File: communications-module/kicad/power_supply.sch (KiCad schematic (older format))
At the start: 25 parts, among them J1 IDC12, P2 USB_A, P3 USB_A, P4 USB_A, P5 BACKUP, U3 TPS2064, U4 PWR_CONN, U5 TPS2064

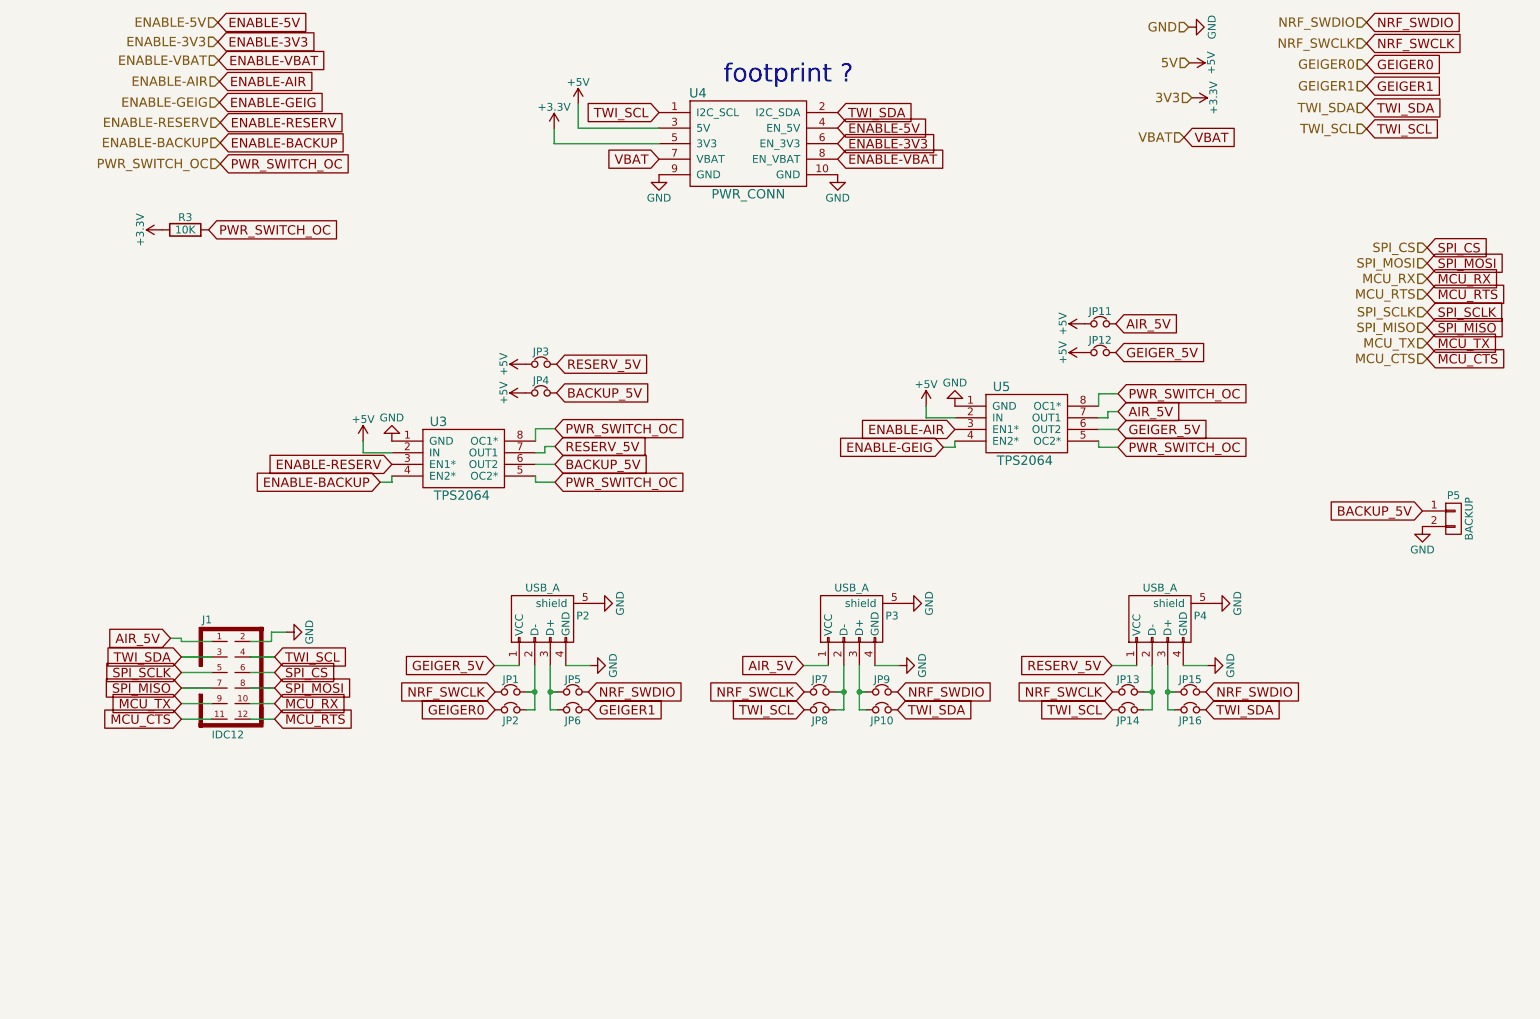
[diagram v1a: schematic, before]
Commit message: Communications Module schematic update
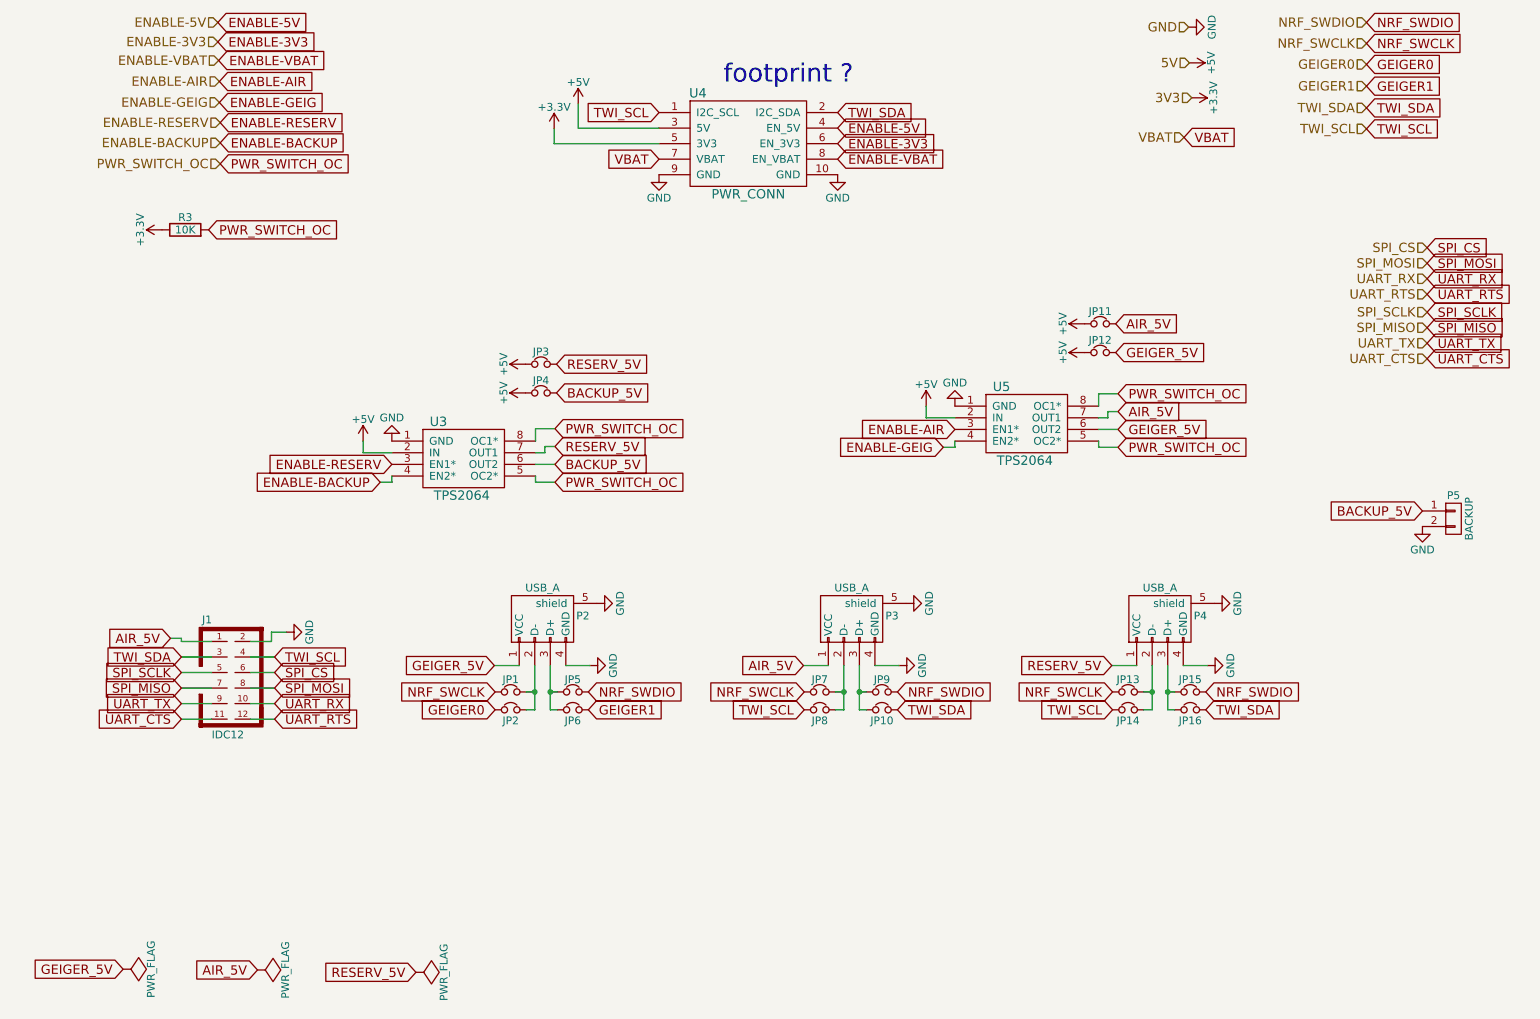
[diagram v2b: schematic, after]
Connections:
- net MCU_CTS renamed UART_CTS
- net MCU_RTS renamed UART_RTS
- net MCU_RX renamed UART_RX
- net MCU_TX renamed UART_TX
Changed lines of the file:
@@
 TWI_SDA
 $Comp
-L GND #PWR019
+L GND #PWR041
 U 1 1 589845A1
 P 4785 2270
-F 0 "#PWR019" H 4785 2020 50  0001 C CNN
+F 0 "#PWR041" H 4785 2020 50  0001 C CNN
 F 1 "GND" H 4785 2120 50  0000 C CNN
 F 2 "" H 4785 2270 60  0000 C CNN
@@
 $EndComp
 $Comp
-L GND #PWR020
+L GND #PWR042
 U 1 1 589845A7
 P 5935 2270
-F 0 "#PWR020" H 5935 2020 50  0001 C CNN
+F 0 "#PWR042" H 5935 2020 50  0001 C CNN
 F 1 "GND" H 5935 2120 50  0000 C CNN
 F 2 "" H 5935 2270 60  0000 C CNN
@@
 $EndComp
 $Comp
-L GND #PWR021
+L GND #PWR043
 U 1 1 589859EA
 P 6375 5030
-F 0 "#PWR021" H 6375 4780 50  0001 C CNN
+F 0 "#PWR043" H 6375 4780 50  0001 C CNN
 F 1 "GND" H 6375 4880 50  0000 C CNN
 F 2 "" H 6375 5030 60  0000 C CNN
@@
 $EndComp
 $Comp
-L GND #PWR022
+L GND #PWR044
 U 1 1 589859F7
 P 8315 5430
-F 0 "#PWR022" H 8315 5180 50  0001 C CNN
+F 0 "#PWR044" H 8315 5180 50  0001 C CNN
 F 1 "GND" H 8315 5280 50  0000 C CNN
 F 2 "" H 8315 5430 60  0000 C CNN
@@
 $EndComp
 $Comp
-L GND #PWR023
+L GND #PWR045
 U 1 1 58985A1D
 P 8360 5030
-F 0 "#PWR023" H 8360 4780 50  0001 C CNN
+F 0 "#PWR045" H 8360 4780 50  0001 C CNN
 F 1 "GND" H 8360 4880 50  0000 C CNN
 F 2 "" H 8360 5030 60  0000 C CNN
@@
 $EndComp
 $Comp
-L GND #PWR024
+L GND #PWR046
 U 1 1 58985A2A
 P 4340 5430
-F 0 "#PWR024" H 4340 5180 50  0001 C CNN
+F 0 "#PWR046" H 4340 5180 50  0001 C CNN
 F 1 "GND" H 4340 5280 50  0000 C CNN
 F 2 "" H 4340 5430 60  0000 C CNN
@@
 $EndComp
 $Comp
-L GND #PWR025
+L GND #PWR047
 U 1 1 58985A50
 P 4385 5030
-F 0 "#PWR025" H 4385 4780 50  0001 C CNN
+F 0 "#PWR047" H 4385 4780 50  0001 C CNN
 F 1 "GND" H 4385 4880 50  0000 C CNN
 F 2 "" H 4385 5030 60  0000 C CNN
@@
 $EndComp
 $Comp
-L GND #PWR026
+L GND #PWR048
 U 1 1 58985A5D
 P 6690 3760
-F 0 "#PWR026" H 6690 3510 50  0001 C CNN
+F 0 "#PWR048" H 6690 3510 50  0001 C CNN
 F 1 "GND" H 6690 3610 50  0000 C CNN
 F 2 "" H 6690 3760 60  0000 C CNN
@@
 	7615 4025 7740 4025
 $Comp
-L GND #PWR027
+L GND #PWR049
 U 1 1 58985A8F
 P 3065 3985
-F 0 "#PWR027" H 3065 3735 50  0001 C CNN
+F 0 "#PWR049" H 3065 3735 50  0001 C CNN
 F 1 "GND" H 3065 3835 50  0000 C CNN
 F 2 "" H 3065 3985 60  0000 C CNN
@@
 RESERV_5V
 $Comp
-L GND #PWR028
+L GND #PWR050
 U 1 1 58985AAE
 P 6330 5430
-F 0 "#PWR028" H 6330 5180 50  0001 C CNN
+F 0 "#PWR050" H 6330 5180 50  0001 C CNN
 F 1 "GND" H 6330 5280 50  0000 C CNN
 F 2 "" H 6330 5430 60  0000 C CNN
@@
 $EndComp
 $Comp
-L +5V #PWR029
+L +5V #PWR051
 U 1 1 58985ABE
 P 3925 3490
-F 0 "#PWR029" H 3925 3340 50  0001 C CNN
+F 0 "#PWR051" H 3925 3340 50  0001 C CNN
 F 1 "+5V" H 3925 3630 50  0000 C CNN
 F 2 "" H 3925 3490 60  0000 C CNN
@@
 $EndComp
 $Comp
-L +5V #PWR030
+L +5V #PWR052
 U 1 1 58985AD9
 P 7525 3230
-F 0 "#PWR030" H 7525 3080 50  0001 C CNN
+F 0 "#PWR052" H 7525 3080 50  0001 C CNN
 F 1 "+5V" H 7525 3370 50  0000 C CNN
 F 2 "" H 7525 3230 60  0000 C CNN
@@
 $EndComp
 $Comp
-L +5V #PWR031
+L +5V #PWR053
 U 1 1 58985AE6
 P 7525 3415
-F 0 "#PWR031" H 7525 3265 50  0001 C CNN
+F 0 "#PWR053" H 7525 3265 50  0001 C CNN
 F 1 "+5V" H 7525 3555 50  0000 C CNN
 F 2 "" H 7525 3415 60  0000 C CNN
@@
 5V
 $Comp
-L +5V #PWR032
+L +5V #PWR054
 U 1 1 58988CC2
 P 8200 1550
-F 0 "#PWR032" H 8200 1400 50  0001 C CNN
+F 0 "#PWR054" H 8200 1400 50  0001 C CNN
 F 1 "+5V" H 8200 1690 50  0000 C CNN
 F 2 "" H 8200 1550 60  0000 C CNN
@@
 $EndComp
 $Comp
-L +3.3V #PWR033
+L +3.3V #PWR055
 U 1 1 58989B65
 P 8215 1775
-F 0 "#PWR033" H 8215 1625 50  0001 C CNN
+F 0 "#PWR055" H 8215 1625 50  0001 C CNN
 F 1 "+3.3V" H 8215 1915 50  0000 C CNN
 F 2 "" H 8215 1775 60  0000 C CNN
@@
 TWI_SCL
 $Comp
-L +5V #PWR034
+L +5V #PWR056
 U 1 1 589845B4
 P 4265 1815
-F 0 "#PWR034" H 4265 1665 50  0001 C CNN
+F 0 "#PWR056" H 4265 1665 50  0001 C CNN
 F 1 "+5V" H 4265 1955 50  0000 C CNN
 F 2 "" H 4265 1815 60  0000 C CNN
@@
 $EndComp
 $Comp
-L +3.3V #PWR035
+L +3.3V #PWR057
 U 1 1 589845AE
 P 4110 1975
-F 0 "#PWR035" H 4110 1825 50  0001 C CNN
+F 0 "#PWR057" H 4110 1825 50  0001 C CNN
 F 1 "+3.3V" H 4110 2115 50  0000 C CNN
 F 2 "" H 4110 1975 60  0000 C CNN
@@
 BACKUP_5V
 $Comp
-L GND #PWR036
+L GND #PWR058
 U 1 1 589977EF
 P 9700 4535
-F 0 "#PWR036" H 9700 4285 50  0001 C CNN
+F 0 "#PWR058" H 9700 4285 50  0001 C CNN
 F 1 "GND" H 9700 4385 50  0000 C CNN
 F 2 "" H 9700 4535 60  0000 C CNN
@@
 AIR_5V
 $Comp
-L GND #PWR037
+L GND #PWR059
 U 1 1 58A00F9B
 P 8195 1320
-F 0 "#PWR037" H 8195 1070 50  0001 C CNN
+F 0 "#PWR059" H 8195 1070 50  0001 C CNN
 F 1 "GND" H 8195 1170 50  0000 C CNN
 F 2 "" H 8195 1320 60  0000 C CNN
@@
 $EndComp
 $Comp
-L +3.3V #PWR038
+L +3.3V #PWR060
 U 1 1 58999FE9
 P 1585 2625
-F 0 "#PWR038" H 1585 2475 50  0001 C CNN
+F 0 "#PWR060" H 1585 2475 50  0001 C CNN
 F 1 "+3.3V" H 1585 2765 50  0000 C CNN
 F 2 "" H 1585 2625 60  0000 C CNN
@@
 SPI_SCLK
 $Comp
-L GND #PWR039
+L GND #PWR061
 U 1 1 58A15D45
 P 2385 5215
-F 0 "#PWR039" H 2385 4965 50  0001 C CNN
+F 0 "#PWR061" H 2385 4965 50  0001 C CNN
 F 1 "GND" H 2385 5065 50  0000 C CNN
 F 2 "" H 2385 5215 60  0000 C CNN
@@
 	1905 5775 1710 5775
 Text GLabel 1710 5675 0    60   Input ~ 0
-MCU_TX
+UART_TX
 Text GLabel 2310 5675 2    60   Input ~ 0
-MCU_RX
+UART_RX
 Text GLabel 1710 5775 0    60   Input ~ 0
-MCU_CTS
+UART_CTS
 Text GLabel 2310 5775 2    60   Input ~ 0
-MCU_RTS
+UART_RTS
 Wire Wire Line
 	2155 5375 2310 5375
@@
 SPI_SCLK
 Text GLabel 9730 3355 2    60   Input ~ 0
-MCU_TX
+UART_TX
 Text GLabel 9730 3455 2    60   Input ~ 0
-MCU_CTS
+UART_CTS
 Text GLabel 9730 2840 2    60   Input ~ 0
 SPI_MOSI
@@
 SPI_CS
 Text GLabel 9730 2940 2    60   Input ~ 0
-MCU_RX
+UART_RX
 Text GLabel 9730 3040 2    60   Input ~ 0
-MCU_RTS
+UART_RTS
 Text HLabel 9730 2740 0    60   Input ~ 0
 SPI_CS
@@
 SPI_MOSI
 Text HLabel 9730 2940 0    60   Input ~ 0
-MCU_RX
+UART_RX
 Text HLabel 9730 3040 0    60   Input ~ 0
-MCU_RTS
+UART_RTS
 Text HLabel 9730 3155 0    60   Input ~ 0
 SPI_SCLK
@@
 SPI_MISO
 Text HLabel 9730 3355 0    60   Input ~ 0
-MCU_TX
+UART_TX
 Text HLabel 9730 3455 0    60   Input ~ 0
-MCU_CTS
+UART_CTS
 Text GLabel 1955 1670 2    60   Input ~ 0
 ENABLE-AIR
 $Comp
-L +5V #PWR040
+L +5V #PWR062
 U 1 1 58985A95
 P 2880 3985
-F 0 "#PWR040" H 2880 3835 50  0001 C CNN
+F 0 "#PWR062" H 2880 3835 50  0001 C CNN
 F 1 "+5V" H 2880 4125 50  0000 C CNN
 F 2 "" H 2880 3985 60  0000 C CNN
@@
 $EndComp
 $Comp
-L +5V #PWR041
+L +5V #PWR063
 U 1 1 58985ACB
 P 3925 3675
-F 0 "#PWR041" H 3925 3525 50  0001 C CNN
+F 0 "#PWR063" H 3925 3525 50  0001 C CNN
 F 1 "+5V" H 3925 3815 50  0000 C CNN
 F 2 "" H 3925 3675 60  0000 C CNN
@@
 BACKUP_5V
 $Comp
-L +5V #PWR042
+L +5V #PWR064
 U 1 1 58985A63
 P 6505 3760
-F 0 "#PWR042" H 6505 3610 50  0001 C CNN
+F 0 "#PWR064" H 6505 3610 50  0001 C CNN
 F 1 "+5V" H 6505 3900 50  0000 C CNN
 F 2 "" H 6505 3760 60  0000 C CNN
@@
 Text Notes 5200 1695 0    118  ~ 0
 footprint ?
+Text GLabel 1335 7385 0    60   Input ~ 0
+GEIGER_5V
+Text GLabel 2200 7390 0    60   Input ~ 0
+AIR_5V
+Text GLabel 3220 7405 0    60   Input ~ 0
+RESERV_5V
+$Comp
+L PWR_FLAG #FLG065
+U 1 1 589AC172
+P 1335 7385
+F 0 "#FLG065" H 1335 7480 50  0001 C CNN
+F 1 "PWR_FLAG" H 1335 7565 50  0000 C CNN
+F 2 "" H 1335 7385 60  0000 C CNN
+F 3 "" H 1335 7385 60  0000 C CNN
+	1    1335 7385
+	0    1    1    0
+$EndComp
+$Comp
+L PWR_FLAG #FLG066
+U 1 1 589AC39B
+P 2200 7390
+F 0 "#FLG066" H 2200 7485 50  0001 C CNN
+F 1 "PWR_FLAG" H 2200 7570 50  0000 C CNN
+F 2 "" H 2200 7390 60  0000 C CNN
+F 3 "" H 2200 7390 60  0000 C CNN
+	1    2200 7390
+	0    1    1    0
+$EndComp
+$Comp
+L PWR_FLAG #FLG067
+U 1 1 589AC824
+P 3220 7405
+F 0 "#FLG067" H 3220 7500 50  0001 C CNN
+F 1 "PWR_FLAG" H 3220 7585 50  0000 C CNN
+F 2 "" H 3220 7405 60  0000 C CNN
+F 3 "" H 3220 7405 60  0000 C CNN
+	1    3220 7405
+	0    1    1    0
+$EndComp
 $EndSCHEMATC
